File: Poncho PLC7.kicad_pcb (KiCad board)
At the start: 4 copper layers, 135.6 x 54.6 mm, 90 parts, among them J1 TB_1X2, J10 Conn_02x12_Odd_Even, J13 Conn_02x05_Odd_Even, J18 Conn_02x05_Odd_Even, J2 TB_1X3-PonchoPLC-rescue, J3 TB_1X2, J4 TB_1X2, J5 TB_1X2, J6 Conn_02x12_Odd_Even, J7 TB_1X2, J9 Conn_02x12_Odd_Even, Q1 FQT13N06L, Q2 FQT13N06L, Q3 FQT13N06L, Q4 FQT13N06L, U1 MCP1416, U2 MCP1416, U3 MCP1416, U4 MCP1416, U5 VO14642AABTR, U6 VO14642AABTR, U7 VO14642AABTR, U8 VO14642AABTR, U9 SI8380P-IU

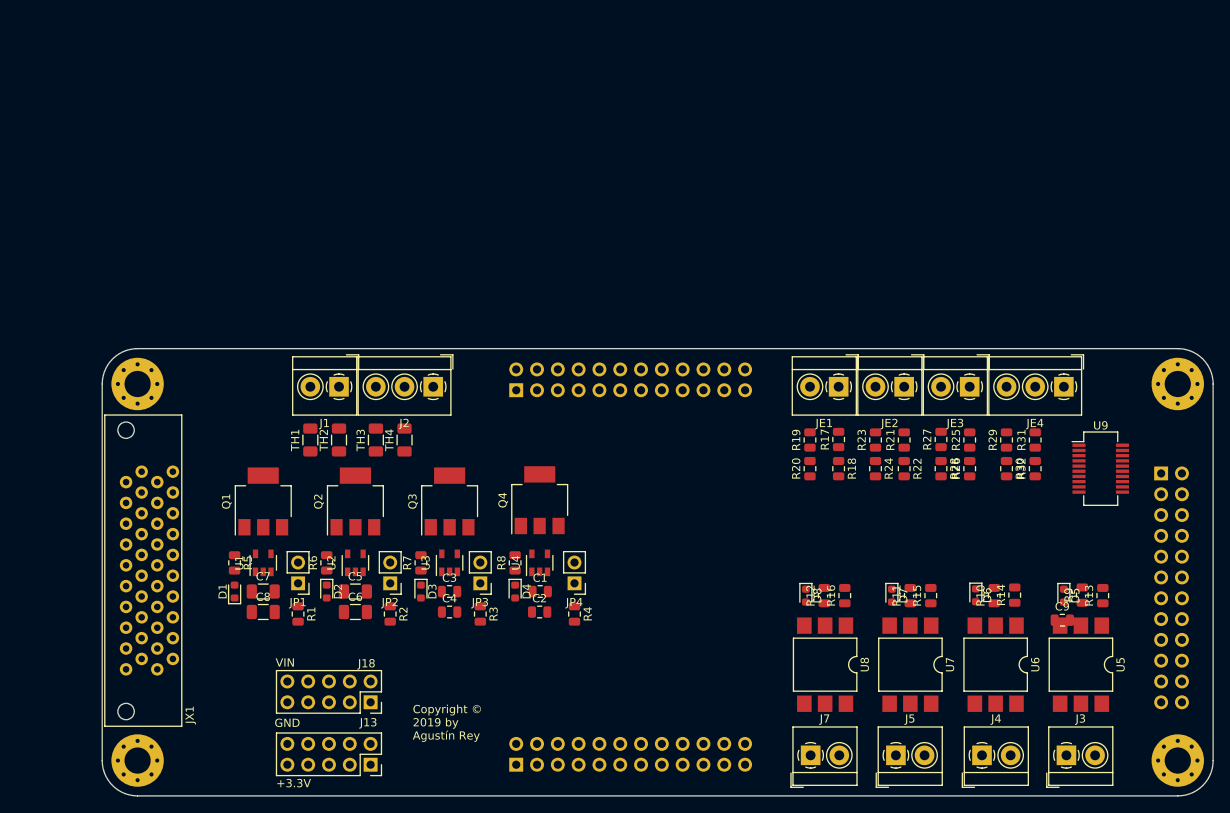
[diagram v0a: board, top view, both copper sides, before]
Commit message: Version 4
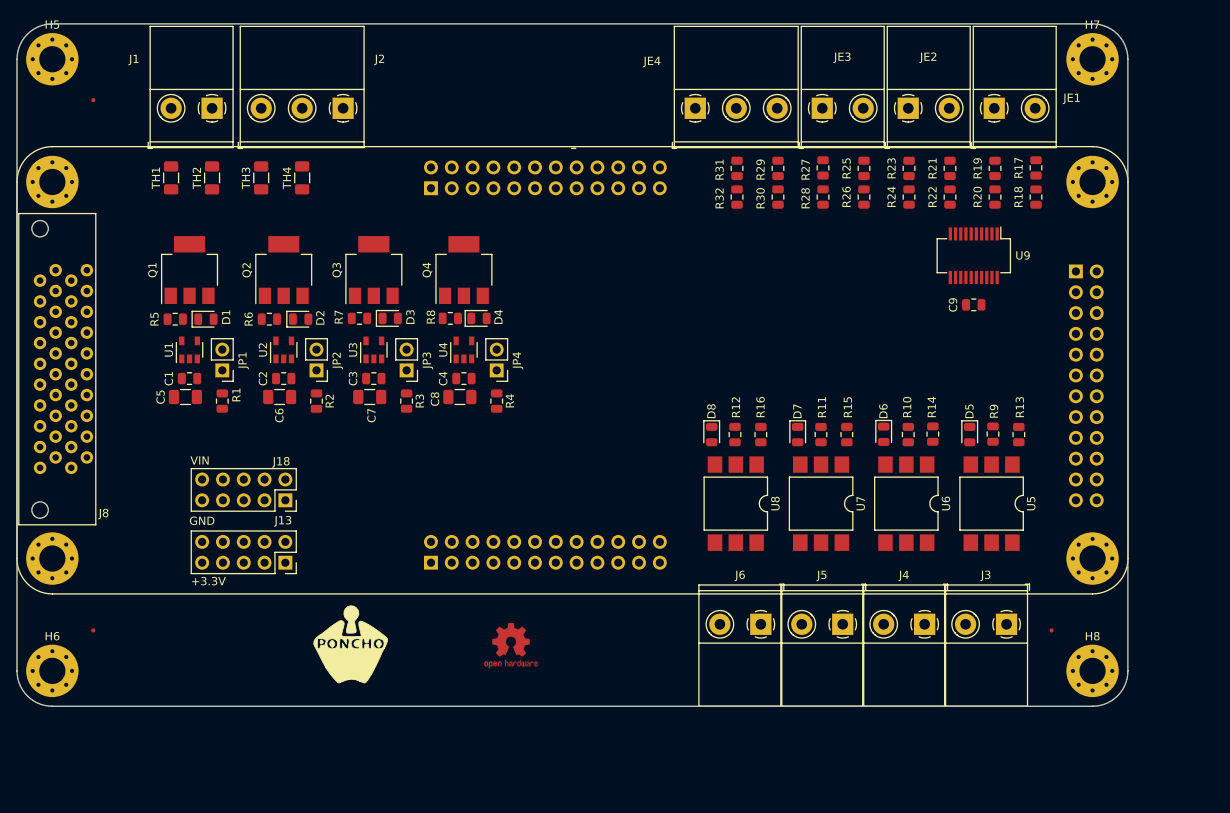
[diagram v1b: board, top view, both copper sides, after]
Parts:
- removed JX1: Conn_02x20_Counter_Clockwise, Poncho-PLC:TX24-40R-LT-H1E
- added  : , Poncho-PLC:Logo_Poncho, F.Cu at (74.4, 136.5)
- added  : , Symbol:OSHW-Logo2_7.3x6mm_Copper, F.Cu at (94.0, 136.6)
- added  : Fiducial, Fiducial:Fiducial_0.5mm_Mask1mm, F.Cu at (43.0, 70.0)
- added  : Fiducial, Fiducial:Fiducial_0.5mm_Mask1mm, F.Cu at (43.0, 134.8)
- added  : Fiducial, Fiducial:Fiducial_0.5mm_Mask1mm, F.Cu at (160.0, 134.8)
- added H5: MountingHole, MountingHole:MountingHole_3.2mm_M3_Pad_Via, F.Cu at (38.0, 65.0)
- added H6: MountingHole, MountingHole:MountingHole_3.2mm_M3_Pad_Via, F.Cu at (38.0, 139.7)
- added H7: MountingHole, MountingHole:MountingHole_3.2mm_M3_Pad_Via, F.Cu at (165.0, 65.0)
- added H8: MountingHole, MountingHole:MountingHole_3.2mm_M3_Pad_Via, F.Cu at (165.0, 139.7)
- added J8: Conn_02x20_Counter_Clockwise, Poncho-PLC:TX24-40R-LT-H1E, F.Cu at (36.5, 114.9)
- D1, D2, D3, D4, D5, D6, D7, D8: footprint LED_SMD:LED_0603_1608Metric -> LED_SMD:LED_0805_2012Metric
- J1: value TB_1X2 -> TB_1X2-PonchoPLC-rescue; footprint Poncho-PLC:TerminalBlock_4Ucon_1x02_P3.50mm_Horizontal -> Poncho-PLC:TerminalBlock_WECO_120-M-311_1x02_P5.00mm_Plug-in_PCB
- J2: footprint Poncho-PLC:TerminalBlock_4Ucon_1x03_P3.50mm_Horizontal -> Poncho-PLC:TerminalBlock_WECO_120-M-311_1x03_P5.00mm_Plug-in_PCB
- J3, J4, J5, JE1, JE2, JE3: footprint Poncho-PLC:TerminalBlock_4Ucon_1x02_P3.50mm_Horizontal -> Poncho-PLC:TerminalBlock_WECO_120-M-311_1x02_P5.00mm_Plug-in_PCB
- J6: value Conn_02x12_Odd_Even -> TB_1X2; footprint Connector_PinSocket_2.54mm:PinSocket_2x12_P2.54mm_Vertical -> Poncho-PLC:TerminalBlock_WECO_120-M-311_1x02_P5.00mm_Plug-in_PCB; moved to F.Cu
- J7: value TB_1X2 -> Conn_02x12_Odd_Even; footprint Poncho-PLC:TerminalBlock_4Ucon_1x02_P3.50mm_Horizontal -> Connector_PinSocket_2.54mm:PinSocket_2x12_P2.54mm_Vertical; moved to B.Cu
- JE4: value TB_1X3-PonchoPLC-rescue -> TB_1X3; footprint Poncho-PLC:TerminalBlock_4Ucon_1x03_P3.50mm_Horizontal -> Poncho-PLC:TerminalBlock_WECO_120-M-311_1x03_P5.00mm_Plug-in_PCB
- R1, R2, R3, R4: value 100k -> 100K
- R17, R19, R21, R23, R25, R27, R29, R31: value 6200 -> 6.2K
- R18, R20, R22, R24, R26, R28, R30, R32: value 2700 -> 2.7K
- moved J7 67.4 mm to (163.0, 90.9), turned to 180 degrees
- moved JE4 56.4 mm to (116.5, 71.0), turned to 0 degrees
- moved J6 52.2 mm to (124.5, 134.0)
- moved C1 50.1 mm to (54.8, 104.0)
- moved R31 49.2 mm to (121.6, 78.3)
- moved R32 49.2 mm to (121.6, 81.8), turned to 270 degrees
- moved R29 43.3 mm to (126.6, 78.3)
- moved R30 43.3 mm to (126.6, 81.8)
- moved C2 42.3 mm to (66.2, 104.0)
- moved R17 41.0 mm to (158.1, 78.3)
- moved R18 41.0 mm to (158.1, 81.8)
- moved R19 40.1 mm to (153.1, 78.3)
- moved R20 40.1 mm to (153.1, 81.8), turned to 270 degrees
- moved C9 40.0 mm to (150.5, 95.0)
- moved JE1 38.9 mm to (153.0, 71.0), turned to 0 degrees
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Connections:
- J6 pad 1: /BaseCIAA7/U1_TX -> Net-(J6-Pad1)
- J6 pad 2: /BaseCIAA7/U1_RX -> Net-(J6-Pad2)
- J7 pad 1: Net-(J7-Pad1) -> /BaseCIAA7/U1_TX
- J7 pad 2: Net-(J7-Pad2) -> /BaseCIAA7/U1_RX
- R17 pad 2: Net-(JE1-Pad1) -> Net-(JE1-Pad2)
- R19 pad 2: Net-(JE1-Pad2) -> Net-(JE1-Pad1)
- R21 pad 2: Net-(JE2-Pad1) -> Net-(JE2-Pad2)
- R23 pad 2: Net-(JE2-Pad2) -> Net-(JE2-Pad1)
- R25 pad 2: Net-(JE3-Pad1) -> Net-(JE3-Pad2)
- R27 pad 2: Net-(JE3-Pad2) -> Net-(JE3-Pad1)
- U5 pad 4: Net-(J3-Pad1) -> Net-(J3-Pad2)
- U5 pad 6: Net-(J3-Pad2) -> Net-(J3-Pad1)
- U6 pad 4: Net-(J4-Pad1) -> Net-(J4-Pad2)
- U6 pad 6: Net-(J4-Pad2) -> Net-(J4-Pad1)
- U7 pad 4: Net-(J5-Pad1) -> Net-(J5-Pad2)
- U7 pad 6: Net-(J5-Pad2) -> Net-(J5-Pad1)
- U8 pad 4: Net-(J7-Pad1) -> Net-(J6-Pad2)
- U8 pad 6: Net-(J7-Pad2) -> Net-(J6-Pad1)
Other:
- board size 135.6 x 54.6 mm -> 135.6 x 83.3 mm
- copper layers 4 -> 2
- net class Default: clearance 0.2 -> 0.3; trace_width 0.25 -> 0.5; via_dia 0.8 -> 1.5; via_drill 0.4 -> 0.7
- net class Delgadas added: clearance 0.3, trace_width 0.3, via_dia 1, via_drill 0.5
- net class Potencia added: clearance 0.3, trace_width 1, via_dia 1, via_drill 0.5
- rule trace_clearance: 0.2 -> 0.3
- rule trace_min: 0.2 -> 0.3
- rule via_min_drill: 0.3 -> 0.5
- rule via_min_size: 0.4 -> 1
- board text added: "Ancho mínimo de pista: 0,25mm Separacion mínima entre pistas: 0,25mm Diametro mínimo de via: 1mm Perforación mínima de via: 0,5m Material de fabricación: FR-4 - 1,6mm Espesor de cobre 35um / 1oz Doble faz con orificios metalizados Terminación superficial SnPb HASL"
- board text added: "Grilla de posicionamiento: Principal 0,5mm Alternativa 0,25mm Grilla de ruteo: Principal 0,5mm Alternativa 0,25mm Referencia: Ernesto Mayer, Estándar 10 mils"
- board text added: "Información de diseño"
- board text added: "Información de fabricación"
- board text removed: "Copyright © 2019 by Agustín Rey"
